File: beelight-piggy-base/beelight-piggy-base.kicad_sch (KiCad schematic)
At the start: 76 parts, among them J1 B_Le, J2 B_Ri, J3 USB_C_Receptacle_PowerOnly_6P, J4 WS2812_ext, J5 PROG, J6 BatSide, J7 DevSide, Q1 AO3400A, SW1 BOOT, U1 MCP73871, U2 BMA253, U3 TPS22917LDBV, U4 ADS1115IDGS, U5 VEML3328, U6 TSOP382xx

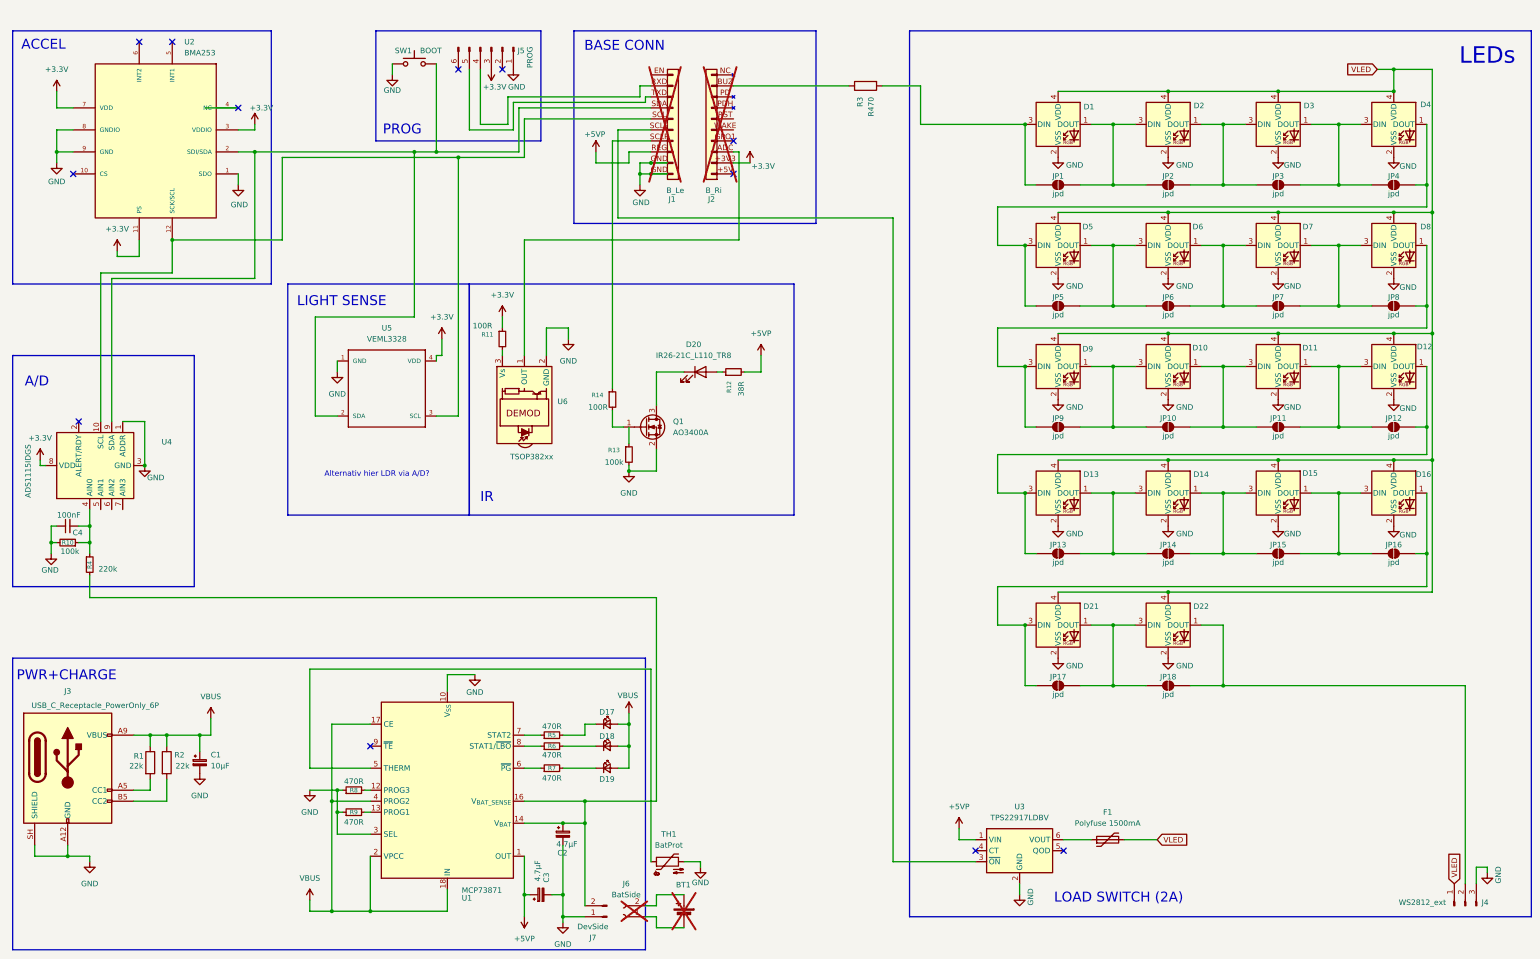
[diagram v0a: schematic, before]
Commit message: first final proto
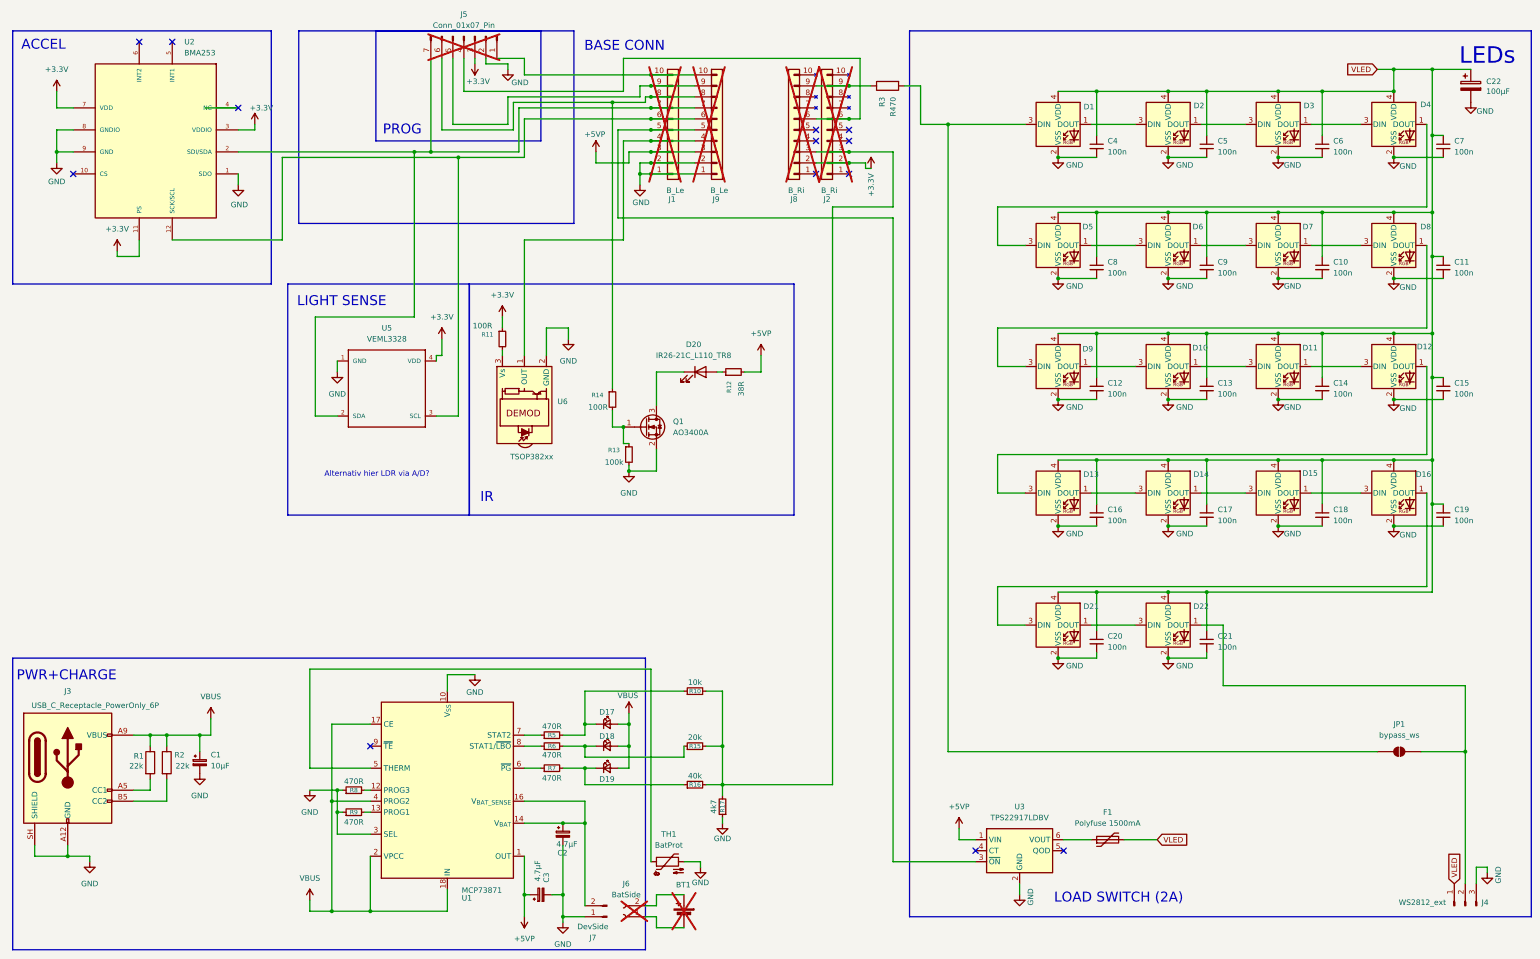
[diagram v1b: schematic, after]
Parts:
- removed J5: PROG, Connector_PinHeader_2.54mm:PinHeader_1x06_P2.54mm_Vertical_SMD_Pin1Right, symbol Connector:Conn_01x06_Pin
- removed JP10, JP11, JP12, JP13, JP14, JP15, JP16, JP17, JP18, JP2, JP3, JP4, JP5, JP6, JP7, JP8, JP9: jpd, symbol Jumper:SolderJumper_2_Open
- removed R4: 220k, symbol Device:R_Small
- removed SW1: BOOT, Button_Switch_SMD:SW_Tactile_SPST_NO_Straight_CK_PTS636Sx25SMTRLFS, symbol Switch:SW_Push
- removed U4: ADS1115IDGS, Package_SO:TSSOP-10_3x3mm_P0.5mm, symbol Analog_ADC:ADS1115IDGS
- added C10, C11, C12, C13, C14, C15, C16, C17, C18, C19, C20, C21, C5, C6, C7, C8, C9: 100n, Capacitor_SMD:C_0402_1005Metric, symbol Device:C_Small
- added C22: 100µF, Capacitor_SMD:C_1210_3225Metric, symbol Device:C_Polarized
- added J5: Conn_01x07_Pin, Connector_PinSocket_2.54mm:PinSocket_1x07_P2.54mm_Vertical, symbol Connector:Conn_01x07_Pin
- added J8: B_Ri, Connector_PinHeader_2.54mm:PinHeader_1x10_P2.54mm_Vertical, symbol Connector_Generic:Conn_01x10
- added J9: B_Le, Connector_PinHeader_2.54mm:PinHeader_1x10_P2.54mm_Vertical, symbol Connector_Generic:Conn_01x10
- added R15: 20k, Resistor_SMD:R_0805_2012Metric, symbol Device:R_Small
- added R16: 40k, Resistor_SMD:R_0805_2012Metric, symbol Device:R_Small
- added R17: 4k7, Resistor_SMD:R_0805_2012Metric, symbol Device:R_Small
- C1, C2, C3: footprint (none) -> Capacitor_SMD:C_1210_3225Metric
- C4: value 100nF -> 100n; footprint (none) -> Capacitor_SMD:C_0402_1005Metric
- D17, D18, D19: footprint (none) -> LED_SMD:LED_0201_0603Metric
- F1: footprint (none) -> Fuse:Fuse_1812_4532Metric
- J1, J2: footprint Connector_PinHeader_2.54mm:PinHeader_1x09_P2.54mm_Vertical -> Connector_PinHeader_2.54mm:PinHeader_1x10_P2.54mm_Vertical
- J3: footprint Connector_USB:USB_C_Receptacle_GCT_USB4105-xx-A_16P_TopMnt_Horizontal -> Connector_USB:USB_C_Receptacle_GCT_USB4125-xx-x-0190_6P_TopMnt_Horizontal
- J4: footprint Connector_Harwin:Harwin_M20-89003xx_1x03_P2.54mm_Horizontal -> Connector_JST:JST_GH_SM03B-GHS-TB_1x03-1MP_P1.25mm_Horizontal
- J7: footprint (none) -> Connector_JST:JST_GH_SM02B-GHS-TB_1x02-1MP_P1.25mm_Horizontal
- JP1: value jpd -> bypass_ws; footprint (none) -> Jumper:SolderJumper-2_P1.3mm_Open_RoundedPad1.0x1.5mm
- R1, R11, R12, R13, R14, R2, R3, R5, R6, R7, R8, R9: footprint (none) -> Resistor_SMD:R_0805_2012Metric
- R10: value 100k -> 10k; footprint (none) -> Resistor_SMD:R_0805_2012Metric
- TH1: footprint Resistor_SMD:R_2816_7142Metric_Pad3.20x4.45mm_HandSolder -> Resistor_SMD:R_0805_2012Metric
- U5: footprint VEML3328:VEML3328 -> beelight:VEML3328
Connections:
- net +3.3V: now also J2.2 (+3V3), J5.3 (Pin_3), J8.2 (+3V3); no longer J2.+3V3 (Pin_2)
- net +5VP: now also J1.3 (REG), J9.3 (REG); no longer J1.REG (Pin_8)
- net GND: now also C4.2, J1.1 (GND), J1.2 (GND), C10.2, C11.2, C12.2, C13.2, C14.2, C15.2, C16.2, C17.2, C18.2, C19.2, C20.2, C21.2, C22.2, C5.2, C6.2, C7.2, C8.2, C9.2, J5.2 (Pin_2), J9.1 (GND), J9.2 (GND), R17.1; no longer C4.1, J1.GND (Pin_10), R10.2
- net VLED: now also C4.1, C10.1, C11.1, C12.1, C13.1, C14.1, C15.1, C16.1, C17.1, C18.1, C19.1, C20.1, C21.1, C22.1, C5.1, C6.1, C7.1, C8.1, C9.1
- net at U2.12 (SCK/SCL), U5.3 (SCL): now also J1.6 (SCL), J9.6 (SCL); no longer J1.SCL (Pin_5)
- net at U3.3 (~{ON}): now also J1.5 (SCL2), J9.5 (SCL2); no longer J1.SCL2 (Pin_6)
- net at R14.1: now also J1.8 (TXD), J5.6 (Pin_6), J9.8 (TXD); no longer J1.SCLP (Pin_7)
- net at U2.2 (SDI/SDA), U5.2 (SDA): now also J1.7 (SDA), J5.7 (Pin_7), J9.7 (SDA); no longer J1.SDA (Pin_4)
- net at D18.1 (K), R6.2: now also R15.1
- net at D1.3 (DIN), R3.2: now also JP1.2 (B); no longer JP1.1 (A)
- net at D1.1 (DOUT), D2.3 (DIN): no longer JP1.2 (B)
- net at D22.1 (DOUT), J4.2 (Pin_2): now also JP1.1 (A)
- net at R13.1: now also Q1.1 (G), R14.2
- net at U6.1 (OUT): now also J1.4 (SCLP), J9.4 (SCLP); no longer J2.ADC (Pin_3)
- net at R3.1: now also J2.9 (BUZ), J8.9 (BUZ); no longer J2.BUZ (Pin_9)
- net at R10.1: now also D17.1 (K), R5.2; no longer C4.2
- net at D19.1 (K), R7.2: now also R16.1
- new net: J1.10 (EN), J5.1 (Pin_1), J9.10 (EN)
- new net: J1.9 (RXD), J5.5 (Pin_5), J9.9 (RXD)
- new net: J2.3 (ADC), J8.3 (ADC), R10.2, R15.2, R16.2, R17.2
- new net: J2.6 (RST), J5.4 (Pin_4), J8.6 (RST)
- no-connect marks 12 -> 13
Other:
- note removed: "A/D"
- moved on the sheet: J2, R3
